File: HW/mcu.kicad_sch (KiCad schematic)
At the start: 12 parts, among them J2 JTAG, SW2 SW_DPST, SW3 SW_DPST, U1 ESP32-S2-MINI-2

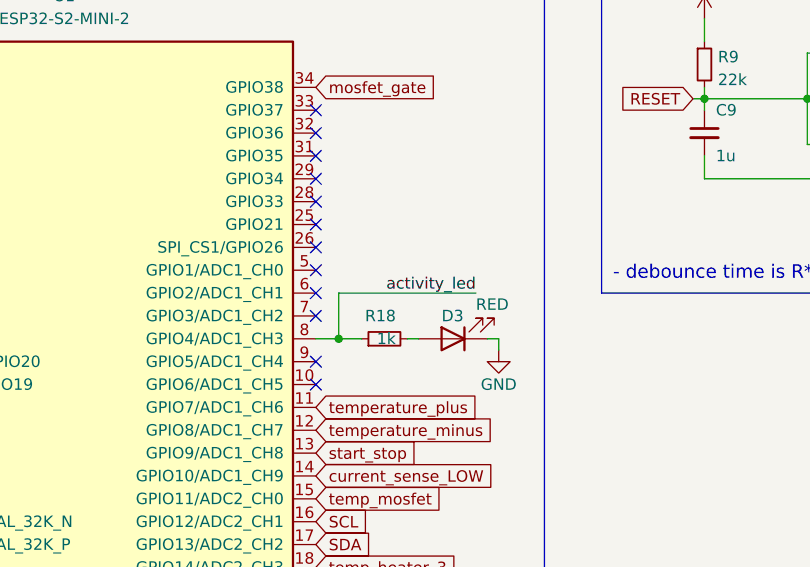
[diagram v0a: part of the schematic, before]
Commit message: revision 0
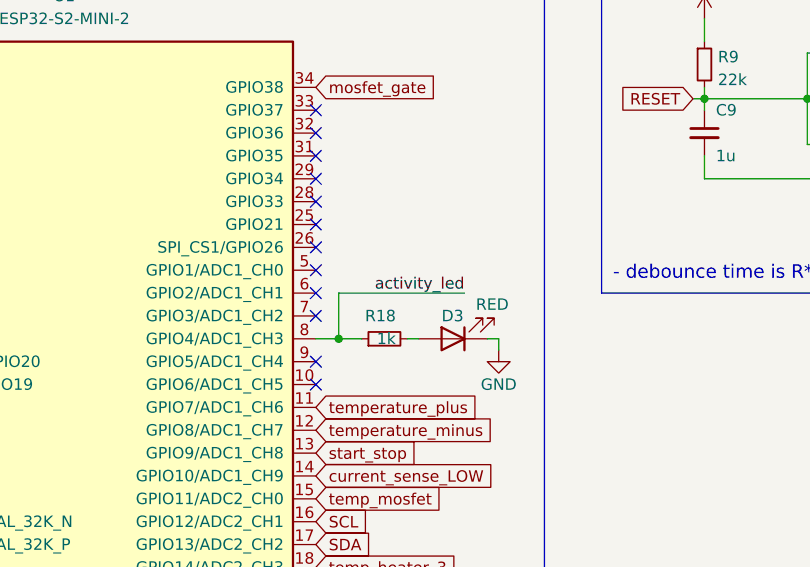
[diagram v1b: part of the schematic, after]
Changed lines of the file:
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@@
     (stroke (width 0) (type default) (color 0 0 0 0))
   )
-  (wire (pts (xy 109.22 62.23) (xy 124.46 62.23))
+  (wire (pts (xy 109.22 62.23) (xy 123.19 62.23))
     (stroke (width 0) (type default) (color 0 0 0 0))
   )
@@
     (effects (font (size 5 5)) (justify left bottom))
   )
-  (label "activity_led" (at 124.46 62.23 180)
+  (label "activity_led" (at 123.19 62.23 180)
     (effects (font (size 1.27 1.27)) (justify right bottom))
   )
